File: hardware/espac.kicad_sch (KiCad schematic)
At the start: 1 part, among them P1 USB_C_Plug

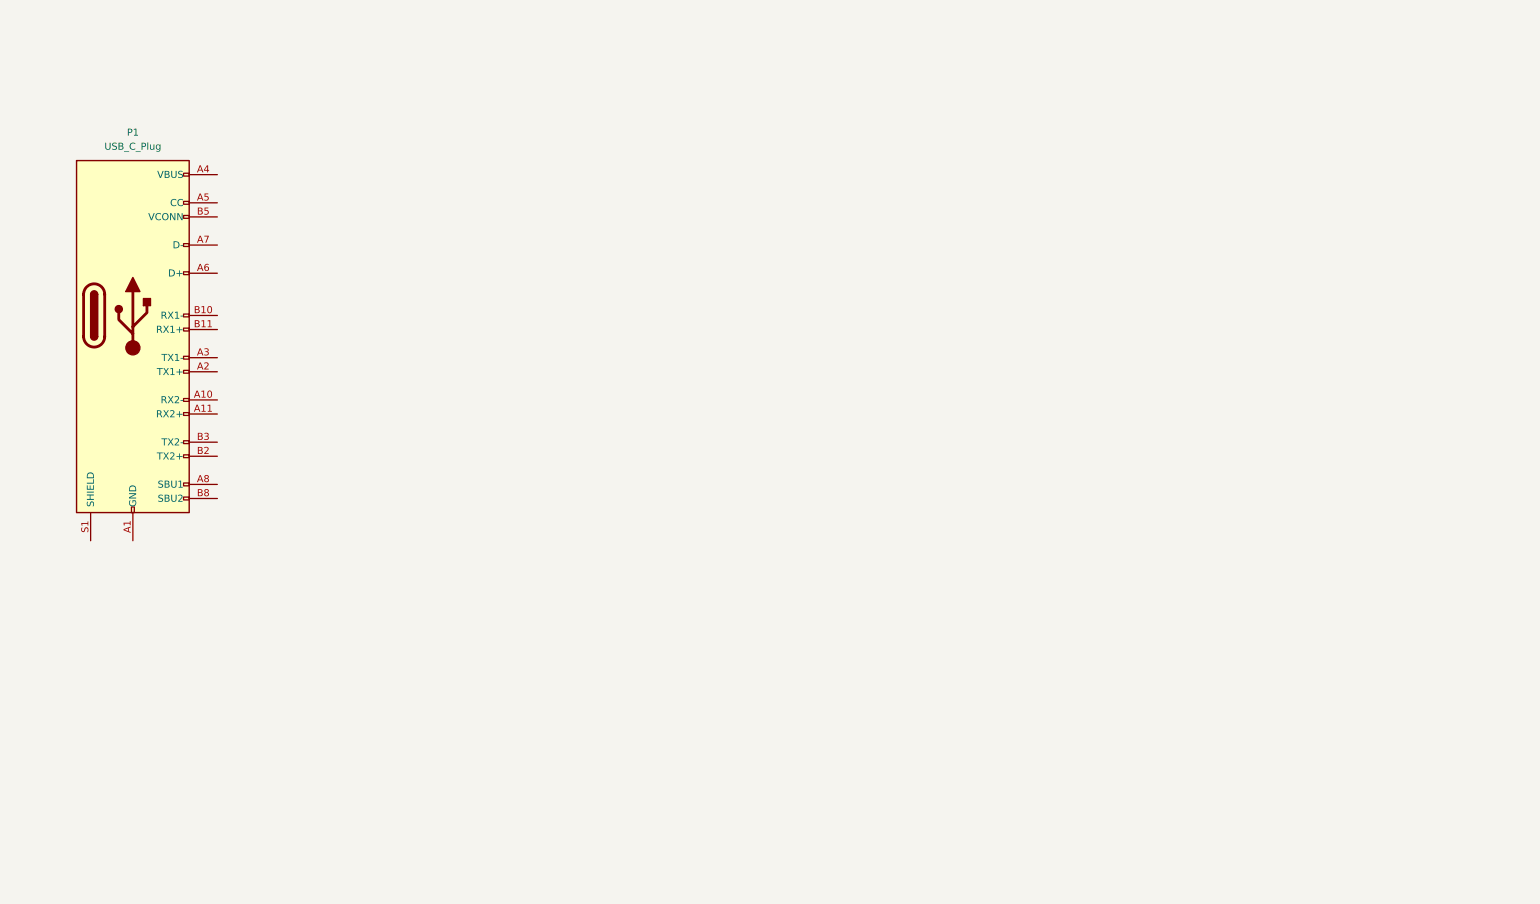
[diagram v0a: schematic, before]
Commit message: feat: schematic files
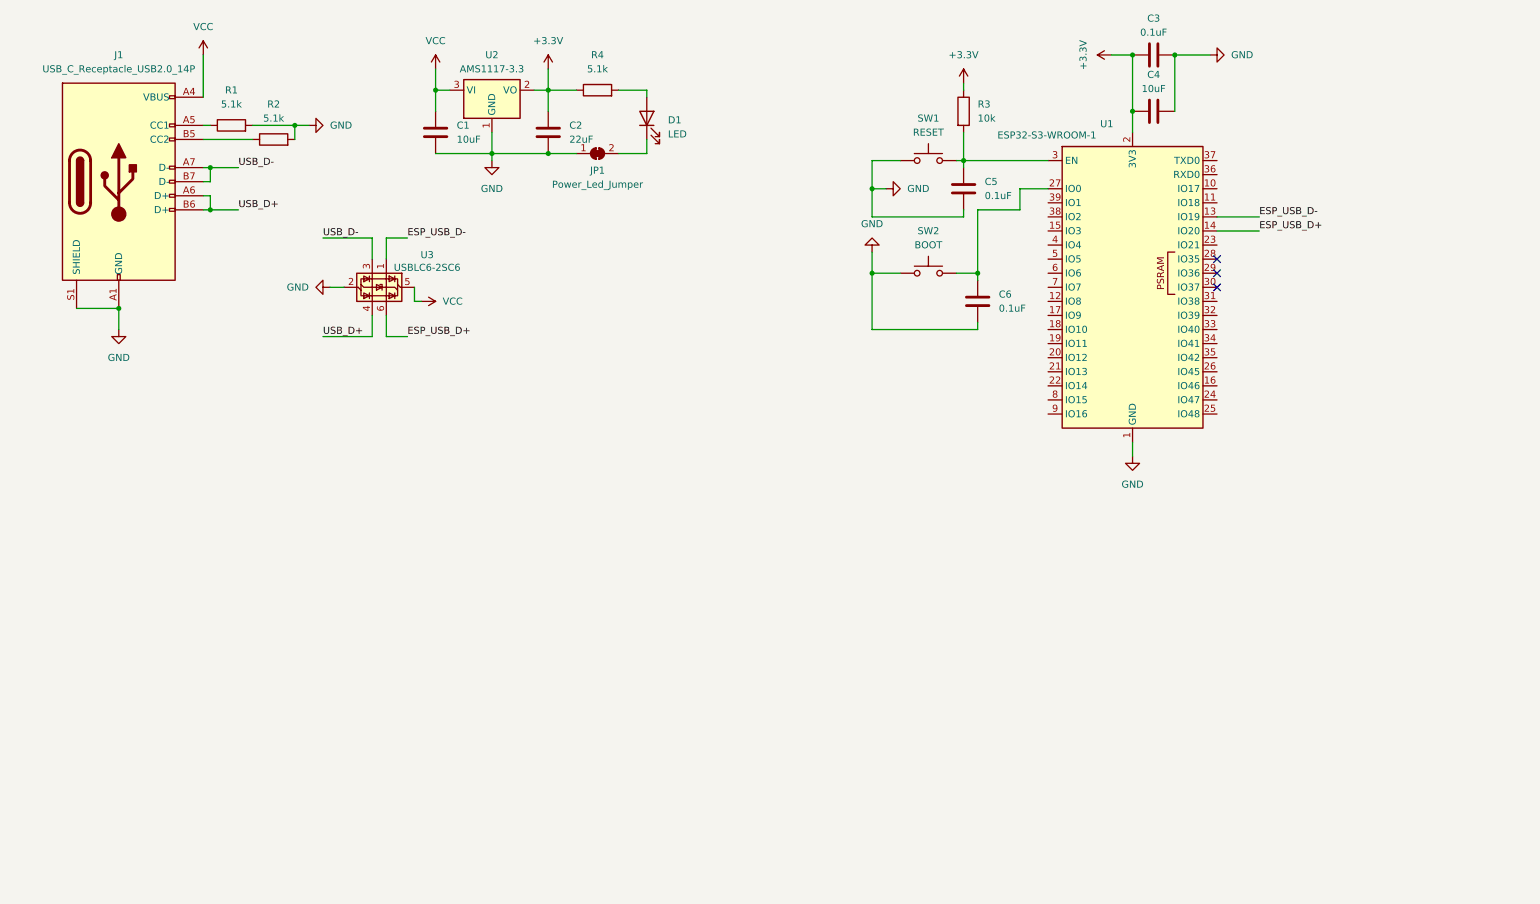
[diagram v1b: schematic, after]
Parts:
- removed P1: USB_C_Plug, Connector_USB:USB_C_Plug_Molex_105444, symbol Connector:USB_C_Plug
- added C1, C4: 10uF, Capacitor_SMD:C_0805_2012Metric_Pad1.18x1.45mm_HandSolder, symbol Device:C
- added C2: 22uF, Capacitor_SMD:C_0805_2012Metric_Pad1.18x1.45mm_HandSolder, symbol Device:C
- added C3, C5, C6: 0.1uF, Capacitor_SMD:C_0805_2012Metric_Pad1.18x1.45mm_HandSolder, symbol Device:C
- added D1: LED, LED_SMD:LED_0603_1608Metric_Pad1.05x0.95mm_HandSolder, symbol Device:LED
- added J1: USB_C_Receptacle_USB2.0_14P, Connector_USB:USB_C_Receptacle_G-Switch_GT-USB-7010ASV, symbol Connector:USB_C_Receptacle_USB2.0_14P
- added JP1: Power_Led_Jumper, Jumper:SolderJumper-2_P1.3mm_Bridged_RoundedPad1.0x1.5mm, symbol Jumper:SolderJumper_2_Bridged
- added R1, R2, R4: 5.1k, Resistor_SMD:R_0805_2012Metric_Pad1.20x1.40mm_HandSolder, symbol Device:R
- added R3: 10k, Resistor_SMD:R_0805_2012Metric_Pad1.20x1.40mm_HandSolder, symbol Device:R
- added SW1: RESET, Button_Switch_SMD:SW_SPST_Omron_B3FS-105xP, symbol Switch:SW_Push
- added SW2: BOOT, Button_Switch_SMD:SW_SPST_Omron_B3FS-105xP, symbol Switch:SW_Push
- added U1: ESP32-S3-WROOM-1, RF_Module:ESP32-S3-WROOM-1, symbol RF_Module:ESP32-S3-WROOM-1
- added U2: AMS1117-3.3, Package_TO_SOT_SMD:SOT-223-3_TabPin2, symbol Regulator_Linear:AMS1117-3.3
- added U3: USBLC6-2SC6, Package_TO_SOT_SMD:SOT-23-6, symbol Power_Protection:USBLC6-2SC6
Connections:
- new net: C5.1, R3.2, SW1.2, U1.3 (EN)
- new net: C6.1, SW2.2, U1.27 (IO0)
- new net: D1.1 (K), JP1.2 (B)
- new net: J1.A5 (CC1), R1.1
- new net: J1.B5 (CC2), R2.1
- new net: D1.2 (A), R4.2
- new net +3.3V: C2.1, C3.1, C4.1, R3.1, R4.1, U1.2 (3V3), U2.2 (VO)
- new net ESP_USB_D+: U1.14 (IO20), U3.6 (I/O1)
- new net ESP_USB_D-: U1.13 (IO19), U3.1 (I/O1)
- new net GND: C1.2, C2.2, C3.2, C4.2, C5.2, C6.2, J1.A1 (GND), J1.A12 (GND), J1.B1 (GND), J1.B12 (GND), J1.S1 (SHIELD), JP1.1 (A), R1.2, R2.2, SW1.1, SW2.1, U1.1 (GND), U1.40 (GND), U1.41 (GND), U2.1 (GND), U3.2 (GND)
- new net USB_D+: J1.A6 (D+), J1.B6 (D+), U3.4 (I/O2)
- new net USB_D-: J1.A7 (D-), J1.B7 (D-), U3.3 (I/O2)
- new net VCC: C1.1, J1.A4 (VBUS), J1.A9 (VBUS), J1.B4 (VBUS), J1.B9 (VBUS), U2.3 (VI), U3.5 (VBUS)
- no-connect marks 0 -> 3

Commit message: chore: pcb stuff
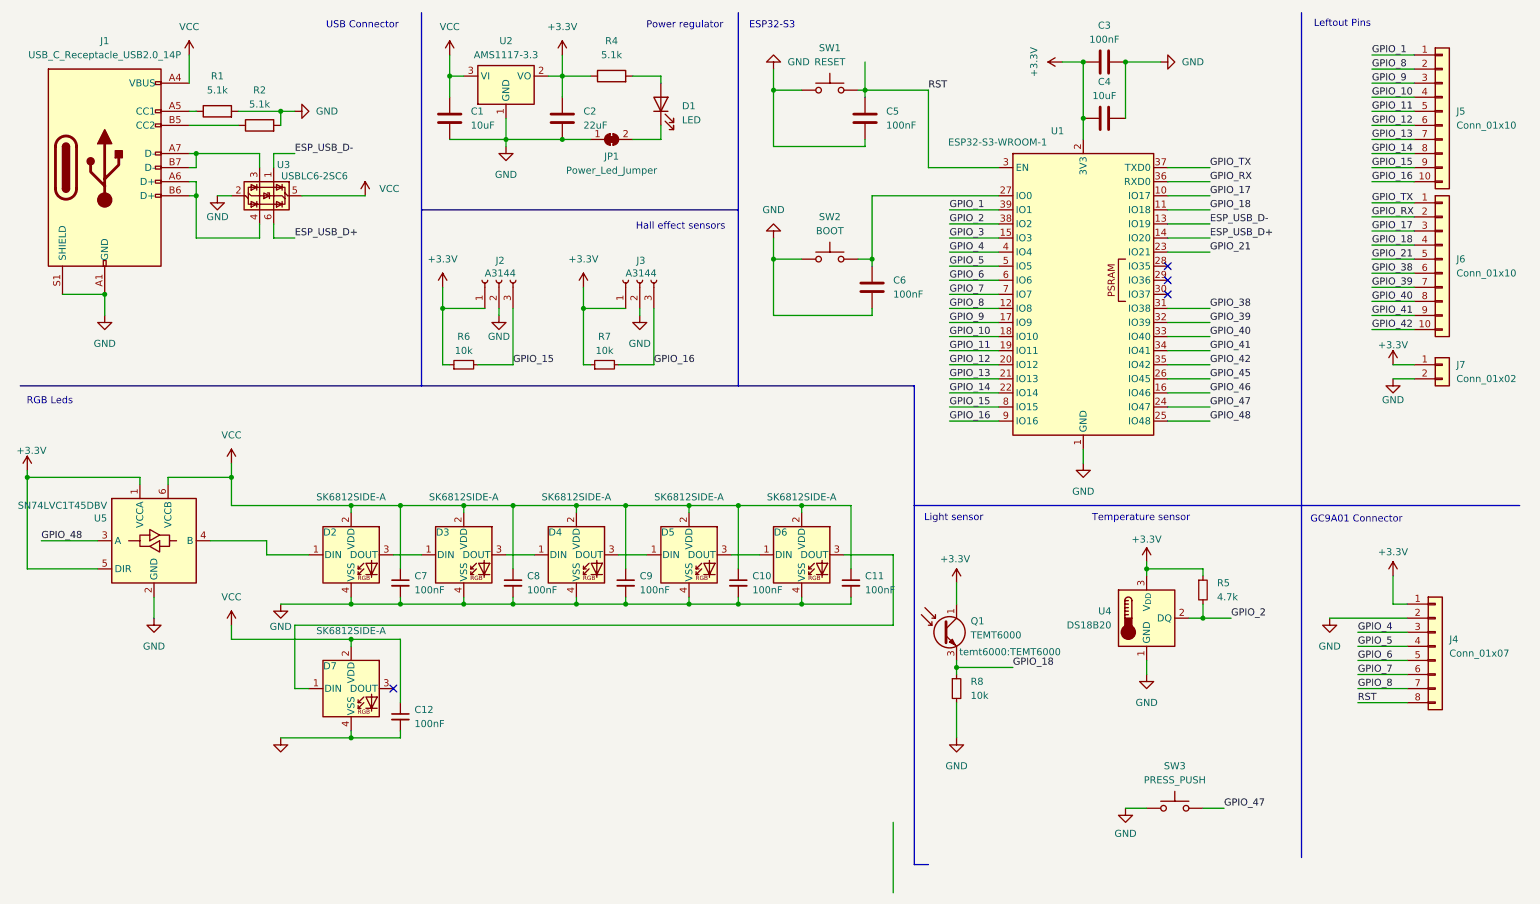
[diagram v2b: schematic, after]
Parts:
- removed R3: 10k, Resistor_SMD:R_0805_2012Metric_Pad1.20x1.40mm_HandSolder, symbol Device:R
- added C10, C11, C12, C7, C8, C9: 100nF, Capacitor_SMD:C_0805_2012Metric_Pad1.18x1.45mm_HandSolder, symbol Device:C_Small
- added D2, D3, D4, D5, D6, D7: SK6812SIDE-A, sk6812:SK6812-SIDE-A, symbol SK6812:SK6812SIDE-A
- added J2, J3: A3144, Connector_JST:JST_GH_SM03B-GHS-TB_1x03-1MP_P1.25mm_Horizontal, symbol Connector:Conn_01x03_Socket
- added J4: Conn_01x07, Connector_FFC-FPC:TE_0-1734839-8_1x08-1MP_P0.5mm_Horizontal, symbol Connector_Generic:Conn_01x08
- added J5, J6: Conn_01x10, Connector_PinSocket_2.54mm:PinSocket_1x10_P2.54mm_Vertical, symbol Connector_Generic:Conn_01x10
- added J7: Conn_01x02, Connector_PinHeader_2.54mm:PinHeader_1x02_P2.54mm_Vertical, symbol Connector_Generic:Conn_01x02
- added Q1: TEMT6000, temt6000:TEMT6000, symbol Sensor_Optical:TEPT4400
- added R5: 4.7k, Resistor_SMD:R_0805_2012Metric_Pad1.20x1.40mm_HandSolder, symbol Device:R_Small
- added R6, R7, R8: 10k, Resistor_SMD:R_0805_2012Metric_Pad1.20x1.40mm_HandSolder, symbol Device:R_Small
- added SW3: PRESS_PUSH, Button_Switch_THT:SW_PUSH-12mm, symbol Switch:SW_Push
- added U4: DS18B20, Package_TO_SOT_THT:TO-92_Inline, symbol Sensor_Temperature:DS18B20
- added U5: SN74LVC1T45DBV, Package_TO_SOT_SMD:SOT-23-6_Handsoldering, symbol Logic_LevelTranslator:SN74LVC1T45DBV
- C3, C5, C6: value 0.1uF -> 100nF
- SW1, SW2: footprint Button_Switch_SMD:SW_SPST_Omron_B3FS-105xP -> Button_Switch_SMD:SW_SPST_FSMSM
- U1: footprint RF_Module:ESP32-S3-WROOM-1 -> PCM_Espressif:ESP32-S3-WROOM-1
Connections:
- net +3.3V: now also J2.1 (Pin_1), J3.1 (Pin_1), J4.1 (Pin_1), J7.1 (Pin_1), Q1.1 (C), R5.1, R6.1, R7.1, U4.3 (V_{DD}), U5.1 (VCCA), U5.5 (DIR)
- net GND: now also C10.2, C11.2, C12.2, C7.2, C8.2, C9.2, D2.4 (VSS), D3.4 (VSS), D4.4 (VSS), D5.4 (VSS), D6.4 (VSS), D7.4 (VSS), J2.2 (Pin_2), J3.2 (Pin_2), J4.2 (Pin_2), J7.2 (Pin_2), R8.2, SW3.1, U4.1 (GND), U5.2 (GND)
- net VCC: now also C10.1, C11.1, C12.1, C7.1, C8.1, C9.1, D2.2 (VDD), D3.2 (VDD), D4.2 (VDD), D5.2 (VDD), D6.2 (VDD), D7.2 (VDD), U5.6 (VCCB)
- net RST: now reaches C5.1, SW1.2, U1.3 (EN)
- net RST: now also J4.8 (Pin_8)
- net GPIO_17: now reaches U1.10 (IO17)
- net GPIO_17: now also J6.3 (Pin_3)
- net GPIO_18: now reaches U1.11 (IO18)
- net GPIO_18: now also J6.4 (Pin_4), Q1.3, R8.1
- net GPIO_8: now reaches U1.12 (IO8)
- net GPIO_8: now also J4.7 (Pin_7), J5.2 (Pin_2)
- net GPIO_3: now reaches U1.15 (IO3)
- net GPIO_46: now reaches U1.16 (IO46)
- net GPIO_9: now reaches U1.17 (IO9)
- net GPIO_9: now also J5.3 (Pin_3)
- net GPIO_10: now reaches U1.18 (IO10)
- net GPIO_10: now also J5.4 (Pin_4)
- net GPIO_11: now reaches U1.19 (IO11)
- net GPIO_11: now also J5.5 (Pin_5)
- net GPIO_12: now reaches U1.20 (IO12)
- net GPIO_12: now also J5.6 (Pin_6)
- net GPIO_13: now reaches U1.21 (IO13)
- net GPIO_13: now also J5.7 (Pin_7)
- net GPIO_14: now reaches U1.22 (IO14)
- net GPIO_14: now also J5.8 (Pin_8)
- net GPIO_21: now reaches U1.23 (IO21)
- net GPIO_21: now also J6.5 (Pin_5)
- net GPIO_47: now reaches U1.24 (IO47)
- net GPIO_47: now also SW3.2
- net GPIO_48: now reaches U1.25 (IO48)
- net GPIO_48: now also U5.3 (A)
- net GPIO_45: now reaches U1.26 (IO45)
- net GPIO_38: now reaches U1.31 (IO38)
- net GPIO_38: now also J6.6 (Pin_6)
- net GPIO_39: now reaches U1.32 (IO39)
- net GPIO_39: now also J6.7 (Pin_7)
- net GPIO_40: now reaches U1.33 (IO40)
- net GPIO_40: now also J6.8 (Pin_8)
- net GPIO_41: now reaches U1.34 (IO41)
- net GPIO_41: now also J6.9 (Pin_9)
- net GPIO_42: now reaches U1.35 (IO42)
- net GPIO_42: now also J6.10 (Pin_10)
- net GPIO_RX: now reaches U1.36 (RXD0)
- net GPIO_RX: now also J6.2 (Pin_2)
- net GPIO_TX: now reaches U1.37 (TXD0)
- net GPIO_TX: now also J6.1 (Pin_1)
- net GPIO_2: now reaches U1.38 (IO2)
- net GPIO_2: now also R5.2, U4.2 (DQ)
- net GPIO_1: now reaches U1.39 (IO1)
- net GPIO_1: now also J5.1 (Pin_1)
- net GPIO_4: now reaches U1.4 (IO4)
- net GPIO_4: now also J4.3 (Pin_3)
- net GPIO_5: now reaches U1.5 (IO5)
- net GPIO_5: now also J4.4 (Pin_4)
- net GPIO_6: now reaches U1.6 (IO6)
- net GPIO_6: now also J4.5 (Pin_5)
- net GPIO_7: now reaches U1.7 (IO7)
- net GPIO_7: now also J4.6 (Pin_6)
- net GPIO_15: now reaches U1.8 (IO15)
- net GPIO_15: now also J2.3 (Pin_3), J5.9 (Pin_9), R6.2
- net GPIO_16: now reaches U1.9 (IO16)
- net GPIO_16: now also J3.3 (Pin_3), J5.10 (Pin_10), R7.2
- net USB_D+: no longer names the net of J1.A6 (D+), J1.B6 (D+), U3.4 (I/O2)
- net USB_D-: no longer names the net of J1.A7 (D-), J1.B7 (D-), U3.3 (I/O2)
- new net: D3.3 (DOUT), D4.1 (DIN)
- new net: D4.3 (DOUT), D5.1 (DIN)
- new net: D2.1 (DIN), U5.4 (B)
- new net: D2.3 (DOUT), D3.1 (DIN)
- new net: D5.3 (DOUT), D6.1 (DIN)
- new net: D6.3 (DOUT), D7.1 (DIN)
- no-connect marks 3 -> 4
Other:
- note added: "ESP32-S3"
- note added: "GC9A01 Connector"
- note added: "Hall effect sensors"
- note added: "Leftout Pins"
- note added: "Light sensor"
- note added: "Power regulator"
- note added: "RGB Leds"
- note added: "Temperature sensor"
- note added: "USB Connector"
- company: (none) -> LunaLabs
- title: (none) -> Espac Schematic
- moved on the sheet: C1, C2, C3, C4, C5, C6, D1, J1, JP1, R1, R2, R4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
